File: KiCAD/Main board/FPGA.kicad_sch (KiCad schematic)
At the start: 2 parts, among them J10 GPIO 0, J11 GPIO 1

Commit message: Worked on main board
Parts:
- J10, J11: footprint Connector_PinHeader_2.54mm:PinHeader_2x20_P2.54mm_Vertical -> Connector_IDC:IDC-Header_2x20_P2.54mm_Vertical
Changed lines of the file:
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@@
       (effects (font (size 1.27 1.27)))
     )
-    (property "Footprint" "Connector_PinHeader_2.54mm:PinHeader_2x20_P2.54mm_Vertical" (at 55.88 63.5 0)
+    (property "Footprint" "Connector_IDC:IDC-Header_2x20_P2.54mm_Vertical" (at 55.88 63.5 0)
       (effects (font (size 1.27 1.27)) hide)
     )
@@
       (effects (font (size 1.27 1.27)))
     )
-    (property "Footprint" "Connector_PinHeader_2.54mm:PinHeader_2x20_P2.54mm_Vertical" (at 110.49 64.77 0)
+    (property "Footprint" "Connector_IDC:IDC-Header_2x20_P2.54mm_Vertical" (at 110.49 64.77 0)
       (effects (font (size 1.27 1.27)) hide)
     )

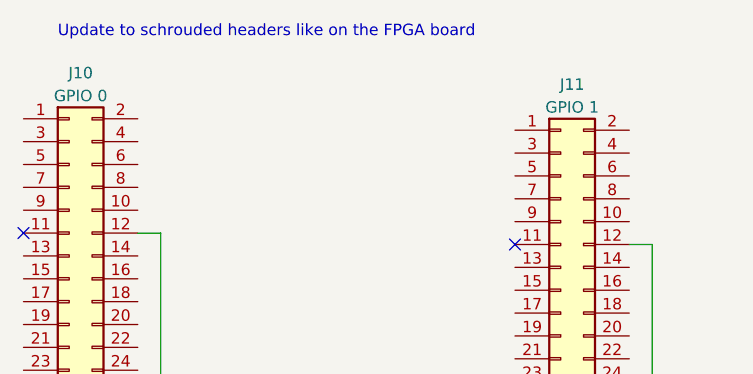
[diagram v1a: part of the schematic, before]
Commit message: Worked on main board
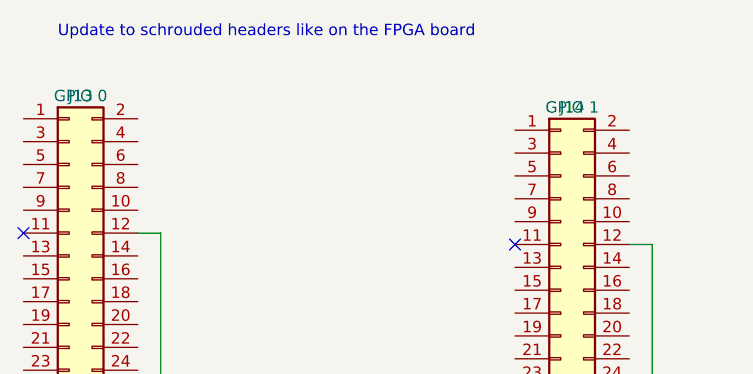
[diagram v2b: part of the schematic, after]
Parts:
- renumbered J10 to J13, J11 to J14
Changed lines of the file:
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@@
   (symbol (lib_id "power:GND") (at 66.04 90.17 0) (unit 1)
     (in_bom yes) (on_board yes) (dnp no) (fields_autoplaced)
-    (property "Reference" "#PWR0101" (at 66.04 96.52 0)
+    (property "Reference" "#PWR0171" (at 66.04 96.52 0)
       (effects (font (size 1.27 1.27)) hide)
     )
@@
       (project "Main board"
         (path "/2f8cbac6-fd11-4240-8e40-3bb6952a0324/22c0a18e-6cf4-4154-962a-243bb7c27459"
-          (reference "#PWR0101") (unit 1)
+          (reference "#PWR0171") (unit 1)
         )
       )
@@
   (symbol (lib_id "Connector_Generic:Conn_02x20_Odd_Even") (at 55.88 63.5 0) (unit 1)
     (in_bom yes) (on_board yes) (dnp no) (fields_autoplaced)
-    (property "Reference" "J10" (at 57.15 35.56 0)
+    (property "Reference" "J13" (at 57.15 38.1 0)
       (effects (font (size 1.27 1.27)))
     )
@@
       (project "Main board"
         (path "/2f8cbac6-fd11-4240-8e40-3bb6952a0324/22c0a18e-6cf4-4154-962a-243bb7c27459"
-          (reference "J10") (unit 1)
+          (reference "J13") (unit 1)
         )
       )
@@
   (symbol (lib_id "Connector_Generic:Conn_02x20_Odd_Even") (at 110.49 64.77 0) (unit 1)
     (in_bom yes) (on_board yes) (dnp no) (fields_autoplaced)
-    (property "Reference" "J11" (at 111.76 36.83 0)
+    (property "Reference" "J14" (at 111.76 39.37 0)
       (effects (font (size 1.27 1.27)))
     )
@@
       (project "Main board"
         (path "/2f8cbac6-fd11-4240-8e40-3bb6952a0324/22c0a18e-6cf4-4154-962a-243bb7c27459"
-          (reference "J11") (unit 1)
+          (reference "J14") (unit 1)
         )
       )
@@
   (symbol (lib_id "power:GND") (at 120.65 91.44 0) (unit 1)
     (in_bom yes) (on_board yes) (dnp no) (fields_autoplaced)
-    (property "Reference" "#PWR0102" (at 120.65 97.79 0)
+    (property "Reference" "#PWR0170" (at 120.65 97.79 0)
       (effects (font (size 1.27 1.27)) hide)
     )
@@
       (project "Main board"
         (path "/2f8cbac6-fd11-4240-8e40-3bb6952a0324/22c0a18e-6cf4-4154-962a-243bb7c27459"
-          (reference "#PWR0102") (unit 1)
+          (reference "#PWR0170") (unit 1)
         )
       )
